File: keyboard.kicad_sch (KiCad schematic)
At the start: 31 parts, among them SW1 SW_PUSH, SW10 SW_PUSH, SW11 SW_PUSH, SW12 SW_PUSH, SW13 SW_PUSH, SW14 SW_PUSH, SW15 SW_PUSH, SW16 SW_PUSH, SW17 SW_PUSH, SW18 SW_PUSH, SW19 SW_PUSH, SW2 SW_PUSH, SW20 SW_PUSH, SW21 SW_PUSH, SW22 SW_PUSH, SW23 SW_PUSH, SW24 SW_PUSH, SW25 SW_PUSH, SW26 SW_PUSH, SW3 SW_PUSH, SW4 SW_PUSH, SW5 SW_PUSH, SW6 SW_PUSH, SW7 SW_PUSH, SW8 SW_PUSH, SW9 SW_PUSH

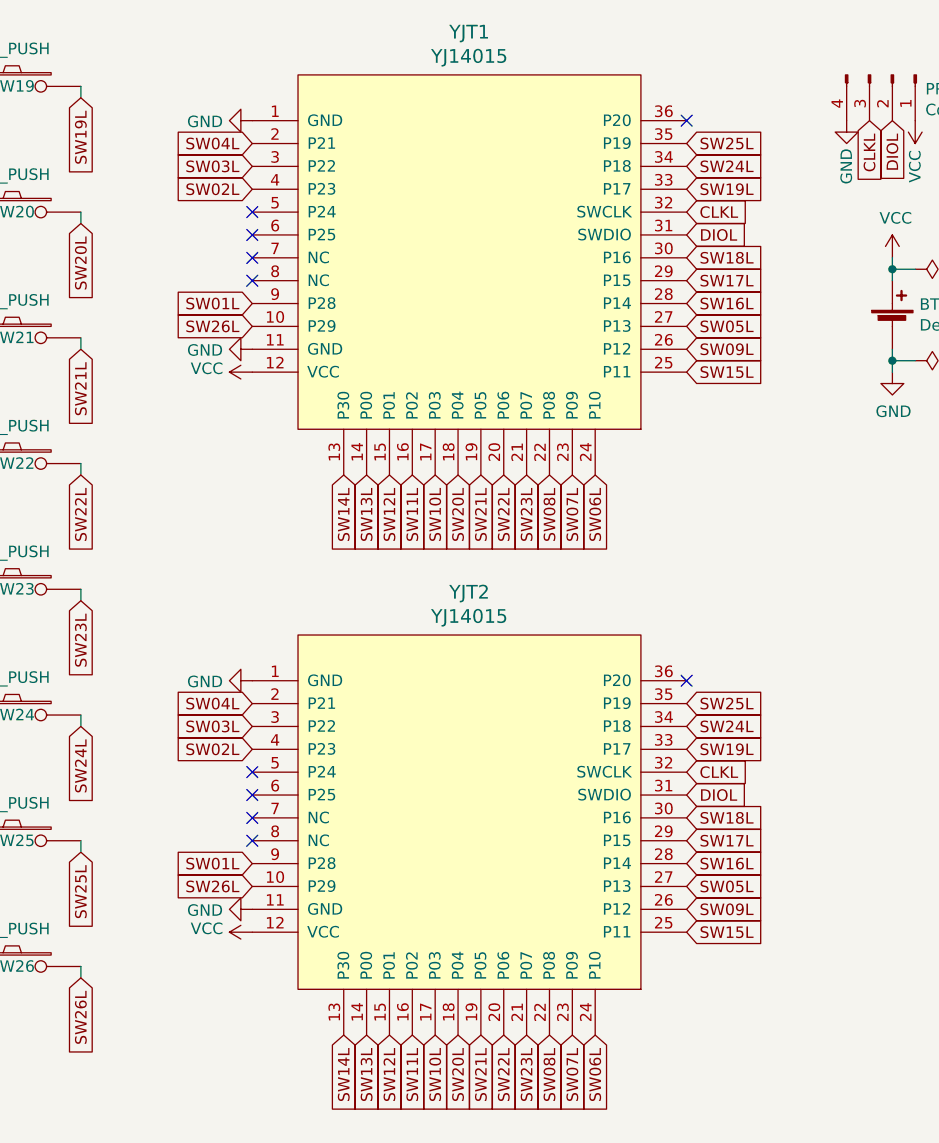
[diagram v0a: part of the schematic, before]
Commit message: Approximate layout
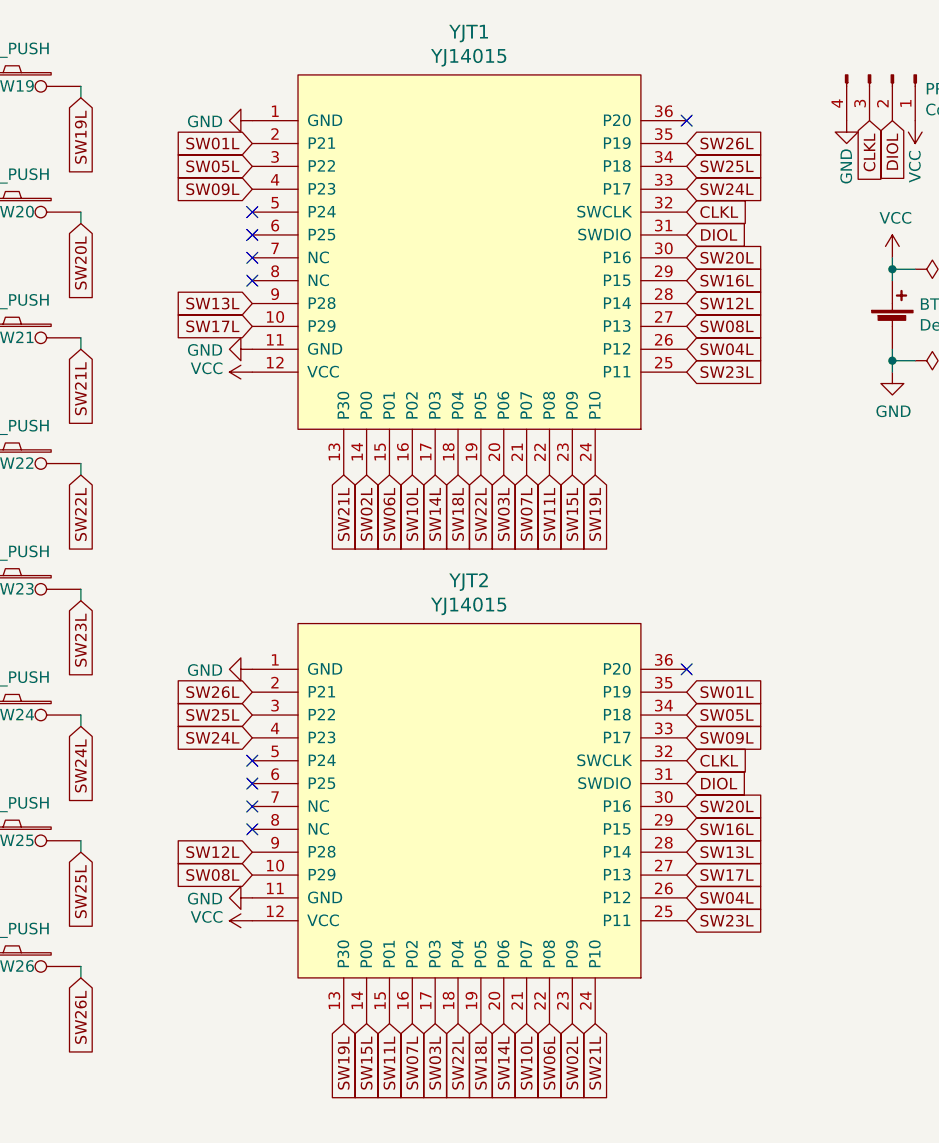
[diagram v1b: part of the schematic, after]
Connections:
- net SW01L: now also YJT1.2 (P21), YJT2.35 (P19); no longer YJT1.9 (P28), YJT2.9 (P28)
- net SW02L: now also YJT1.14 (P00), YJT2.23 (P09); no longer YJT1.4 (P23), YJT2.4 (P23)
- net SW03L: now also YJT1.20 (P06), YJT2.17 (P03); no longer YJT1.3 (P22), YJT2.3 (P22)
- net SW04L: now also YJT1.26 (P12), YJT2.26 (P12); no longer YJT1.2 (P21), YJT2.2 (P21)
- net SW05L: now also YJT1.3 (P22), YJT2.34 (P18); no longer YJT1.27 (P13), YJT2.27 (P13)
- net SW06L: now also YJT1.15 (P01), YJT2.22 (P08); no longer YJT1.24 (P10), YJT2.24 (P10)
- net SW07L: now also YJT1.21 (P07), YJT2.16 (P02); no longer YJT1.23 (P09), YJT2.23 (P09)
- net SW08L: now also YJT1.27 (P13), YJT2.10 (P29); no longer YJT1.22 (P08), YJT2.22 (P08)
- net SW09L: now also YJT1.4 (P23), YJT2.33 (P17); no longer YJT1.26 (P12), YJT2.26 (P12)
- net SW10L: now also YJT1.16 (P02), YJT2.21 (P07); no longer YJT1.17 (P03), YJT2.17 (P03)
- net SW11L: now also YJT1.22 (P08), YJT2.15 (P01); no longer YJT1.16 (P02), YJT2.16 (P02)
- net SW12L: now also YJT1.28 (P14), YJT2.9 (P28); no longer YJT1.15 (P01), YJT2.15 (P01)
- net SW13L: now also YJT1.9 (P28), YJT2.28 (P14); no longer YJT1.14 (P00), YJT2.14 (P00)
- net SW14L: now also YJT1.17 (P03), YJT2.20 (P06); no longer YJT1.13 (P30), YJT2.13 (P30)
- net SW15L: now also YJT1.23 (P09), YJT2.14 (P00); no longer YJT1.25 (P11), YJT2.25 (P11)
- net SW16L: now also YJT1.29 (P15), YJT2.29 (P15); no longer YJT1.28 (P14), YJT2.28 (P14)
- net SW17L: now also YJT1.10 (P29), YJT2.27 (P13); no longer YJT1.29 (P15), YJT2.29 (P15)
- net SW18L: now also YJT1.18 (P04), YJT2.19 (P05); no longer YJT1.30 (P16), YJT2.30 (P16)
- net SW19L: now also YJT1.24 (P10), YJT2.13 (P30); no longer YJT1.33 (P17), YJT2.33 (P17)
- net SW20L: now also YJT1.30 (P16), YJT2.30 (P16); no longer YJT1.18 (P04), YJT2.18 (P04)
- net SW21L: now also YJT1.13 (P30), YJT2.24 (P10); no longer YJT1.19 (P05), YJT2.19 (P05)
- net SW22L: now also YJT1.19 (P05), YJT2.18 (P04); no longer YJT1.20 (P06), YJT2.20 (P06)
- net SW23L: now also YJT1.25 (P11), YJT2.25 (P11); no longer YJT1.21 (P07), YJT2.21 (P07)
- net SW24L: now also YJT1.33 (P17), YJT2.4 (P23); no longer YJT1.34 (P18), YJT2.34 (P18)
- net SW25L: now also YJT1.34 (P18), YJT2.3 (P22); no longer YJT1.35 (P19), YJT2.35 (P19)
- net SW26L: now also YJT1.35 (P19), YJT2.2 (P21); no longer YJT1.10 (P29), YJT2.10 (P29)
